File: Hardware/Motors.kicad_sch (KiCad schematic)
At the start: 6 parts, among them J12 Motor, U9 L298N

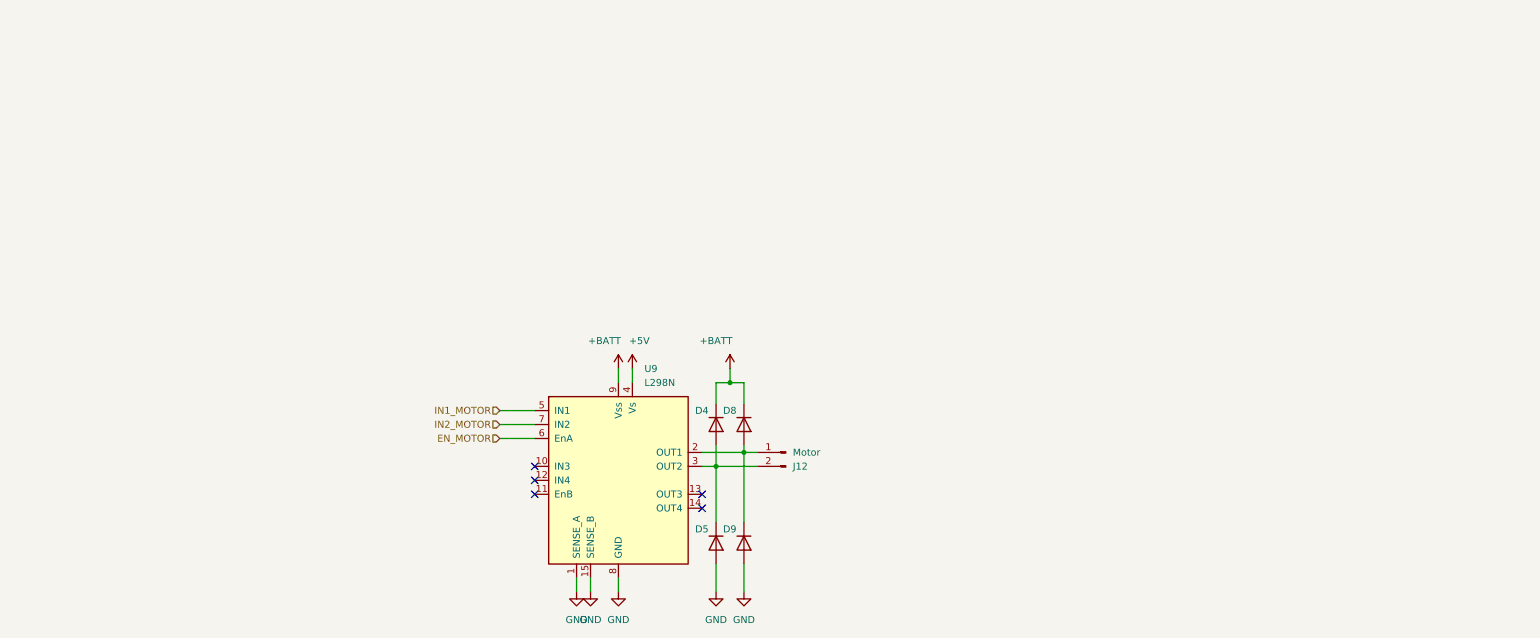
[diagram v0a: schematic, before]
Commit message: Update of PCB
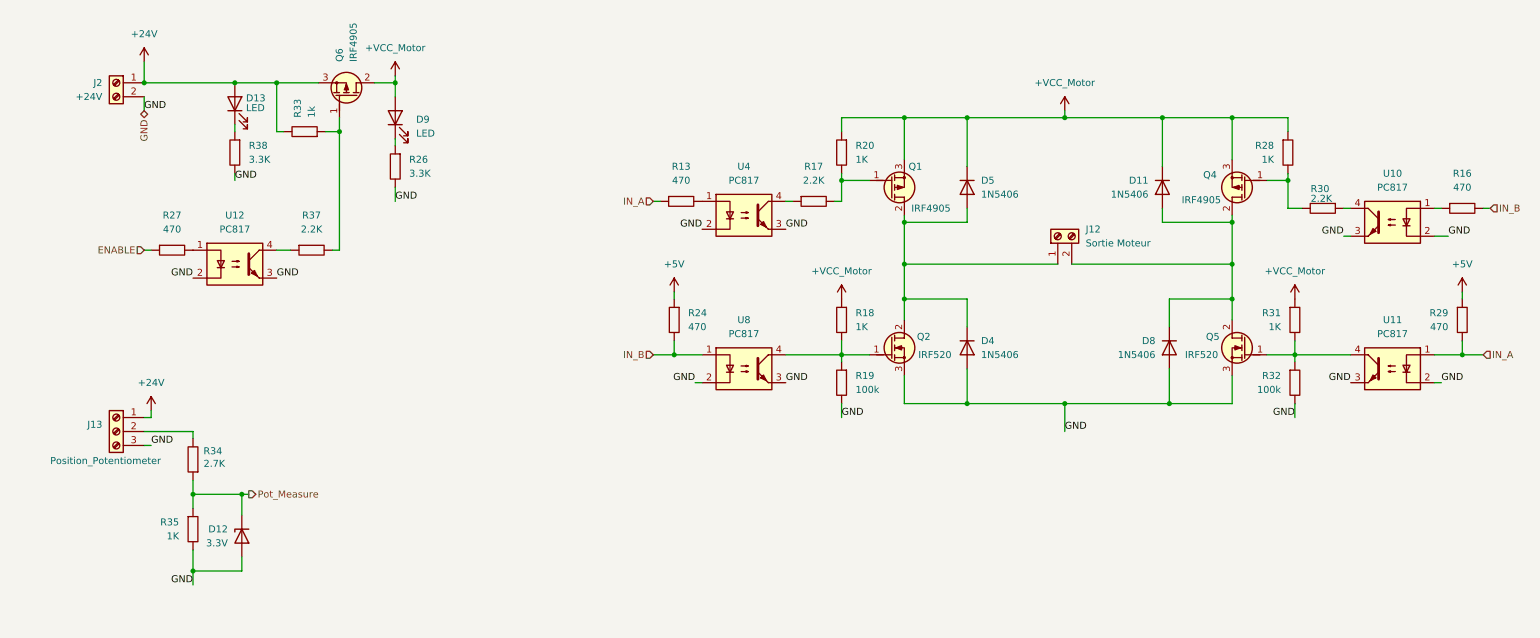
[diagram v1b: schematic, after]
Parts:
- removed D4, D5, D8, D9: 1N4148, Diode_THT:D_DO-35_SOD27_P7.62mm_Horizontal, symbol Diode:1N4148
- removed J12: Motor, TerminalBlock_Phoenix:TerminalBlock_Phoenix_MKDS-1,5-2-5.08_1x02_P5.08mm_Horizontal, symbol Connector:Conn_01x02_Pin
- removed U9: L298N, Package_TO_SOT_THT:TO-220-15_P2.54x2.54mm_StaggerOdd_Lead4.58mm_Vertical, symbol Driver_Motor:L298N
- added D11, D4, D5, D8: 1N5406, Diode_THT:D_DO-201AD_P15.24mm_Horizontal, symbol Diode:1N5406
- added D12: 3.3V, Diode_THT:D_A-405_P10.16mm_Horizontal, symbol Device:D_Zener
- added D13, D9: LED, LED_THT:LED_D3.0mm, symbol Device:LED
- added J12: Sortie Moteur, TerminalBlock_Phoenix:TerminalBlock_Phoenix_MKDS-1,5-2-5.08_1x02_P5.08mm_Horizontal, symbol Connector:Screw_Terminal_01x02
- added J13: Position_Potentiometer, TerminalBlock_Phoenix:TerminalBlock_Phoenix_MKDS-1,5-3-5.08_1x03_P5.08mm_Horizontal, symbol Connector:Screw_Terminal_01x03
- added J2: +24V, TerminalBlock_Phoenix:TerminalBlock_Phoenix_MKDS-1,5-2-5.08_1x02_P5.08mm_Horizontal, symbol Connector:Screw_Terminal_01x02
- added Q1, Q4, Q6: IRF4905, Package_TO_SOT_THT:TO-220-3_Vertical, symbol PCM_Transistor_MOSFET_AKL:IRF4905
- added Q2, Q5: IRF520, Package_TO_SOT_THT:TO-220-3_Vertical, symbol PCM_Transistor_MOSFET_AKL:IRF520
- added R13, R16, R24, R27, R29: 470, Resistor_THT:R_Axial_DIN0207_L6.3mm_D2.5mm_P7.62mm_Horizontal, symbol PCM_SL_Devices:Resistor_0.5W
- added R17, R30, R37: 2.2K, Resistor_THT:R_Axial_DIN0207_L6.3mm_D2.5mm_P7.62mm_Horizontal, symbol PCM_SL_Devices:Resistor_0.5W
- added R18, R20, R28, R31: 1K, Resistor_THT:R_Axial_DIN0207_L6.3mm_D2.5mm_P7.62mm_Horizontal, symbol PCM_SL_Devices:Resistor_0.5W
- added R19, R32: 100k, Resistor_THT:R_Axial_DIN0207_L6.3mm_D2.5mm_P7.62mm_Horizontal, symbol PCM_SL_Devices:Resistor_0.5W
- added R26, R38: 3.3K, Resistor_THT:R_Axial_DIN0207_L6.3mm_D2.5mm_P7.62mm_Horizontal, symbol PCM_SL_Devices:Resistor_0.5W
- added R33: 1k, Resistor_THT:R_Axial_DIN0207_L6.3mm_D2.5mm_P7.62mm_Horizontal, symbol PCM_SL_Devices:Resistor_0.5W
- added R34: 2.7K, Resistor_THT:R_Axial_DIN0207_L6.3mm_D2.5mm_P7.62mm_Horizontal, symbol PCM_SL_Devices:Resistor
- added R35: 1K, Resistor_THT:R_Axial_DIN0207_L6.3mm_D2.5mm_P7.62mm_Horizontal, symbol PCM_SL_Devices:Resistor
- added U10, U11, U12, U4, U8: PC817, Package_DIP:DIP-4_W7.62mm, symbol Isolator:PC817
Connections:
- net +5V: now also R24.1, R29.1
- net GND: now also D12.2 (A), D4.2 (A), D8.2 (A), J13.3 (Pin_3), J2.2 (Pin_2), Q2.3 (S), Q5.3 (S), R19.2, R26.2, R32.2, R35.2, R38.2, U10.2, U10.3, U11.2, U11.3, U12.2, U12.3, U4.2, U4.3, U8.2, U8.3
- new net: R27.2, U12.1
- new net: D4.1 (K), D5.2 (A), J12.1 (Pin_1), Q1.2 (D), Q2.2 (D)
- new net: Q1.1 (G), R17.2, R20.2
- new net: Q5.1 (G), R31.2, R32.1, U11.4
- new net: D11.2 (A), D8.1 (K), J12.2 (Pin_2), Q4.2 (D), Q5.2 (D)
- new net: R37.1, U12.4
- new net: Q6.1 (G), R33.1, R37.2
- new net: D9.1 (K), R26.1
- new net: R13.2, U4.1
- new net: R17.1, U4.4
- new net: Q4.1 (G), R28.2, R30.2
- new net: Q2.1 (G), R18.2, R19.1, U8.4
- new net: R16.1, U10.1
- new net: D13.1 (K), R38.1
- new net: J13.2 (Pin_2), R34.2
- new net: R30.1, U10.4
- new net +24V: D13.2 (A), J13.1 (Pin_1), J2.1 (Pin_1), Q6.3 (S), R33.2
- new net +VCC_Motor: D11.1 (K), D5.1 (K), D9.2 (A), Q1.3 (S), Q4.3 (S), Q6.2 (D), R18.1, R20.1, R28.1, R31.1
- new net ENABLE: R27.1
- new net IN_A: R13.1, R29.2, U11.1
- new net IN_B: R16.2, R24.2, U8.1
- new net Pot_Measure: D12.1 (K), R34.1, R35.1
- no-connect marks 5 -> 0
